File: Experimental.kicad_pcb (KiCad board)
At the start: 4 copper layers, 50.5 x 71 mm, 64 parts, among them J1 3v3 Terminal, J2 Screw_Terminal, J3 Screw_Terminal_4x, J4 Screw_Terminal_4x, J5 -/+ LIPO PIN, J6 Screw_Terminal, J7 20279-001E-03, J8 GND Terminal, Q1 AO3400A, Q2_32mW1 AO3400A, Q4 AO3400A, U6 NEO-6M-GPS

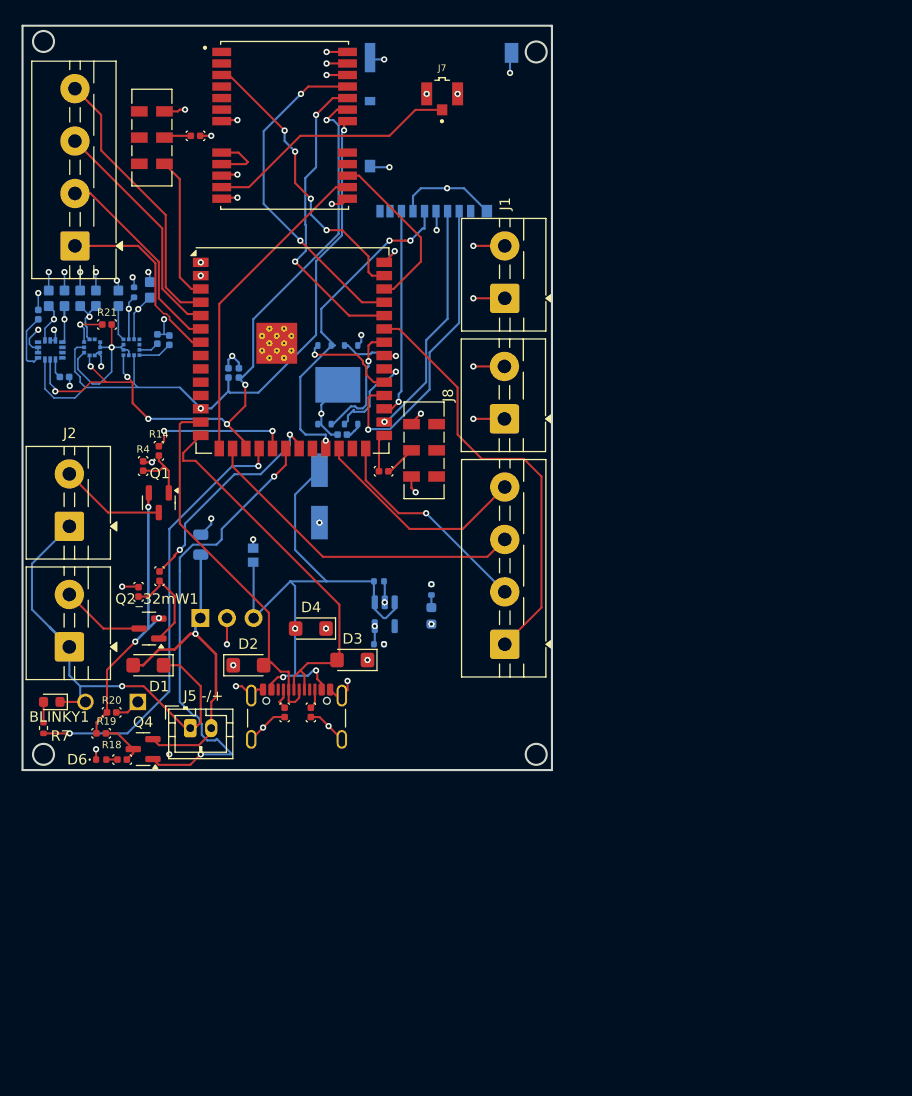
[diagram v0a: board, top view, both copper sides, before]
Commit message: Version 4.0
Schematic Cleanup and PCB Layout/Impletementation
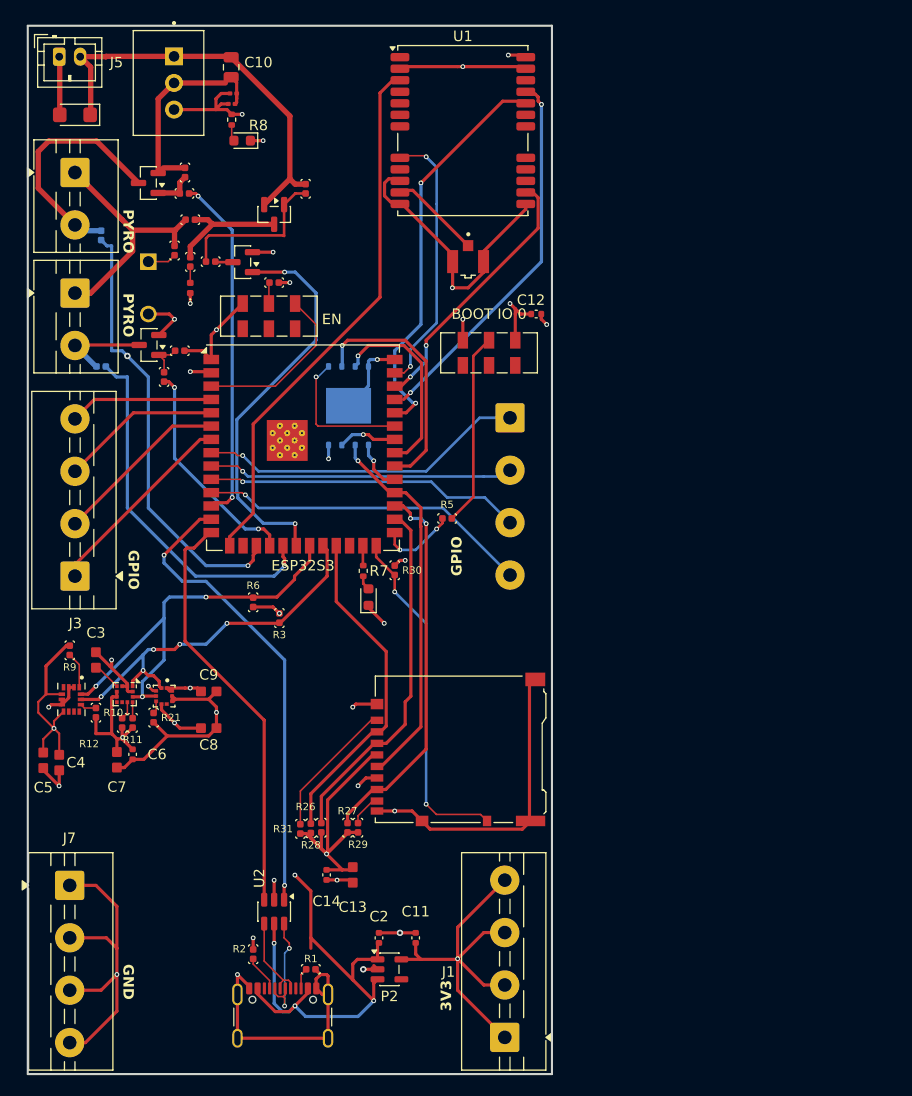
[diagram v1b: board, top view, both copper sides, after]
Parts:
- removed 5v1: LP5907MFX-3.3, Package_TO_SOT_SMD:SOT-23-5
- removed BLINKY1: GREEN LED, LED_SMD:LED_0603_1608Metric
- removed D3: SMF6V0A, Diode_SMD:D_SMF
- removed D4: SMF6V5A, Diode_SMD:D_SMF
- removed D6: RED LED, LED_SMD:LED_0402_1005Metric
- removed J4: Screw_Terminal_4x, TerminalBlock:TerminalBlock_MaiXu_MX126-5.0-04P_1x04_P5.00mm
- removed J5 -/+: LIPO PIN, Connector_JST:JST_PH_B2B-PH-K_1x02_P2.00mm_Vertical
- removed J6: Screw_Terminal, TerminalBlock:TerminalBlock_MaiXu_MX126-5.0-02P_1x02_P5.00mm
- removed J8: GND Terminal, TerminalBlock:TerminalBlock_MaiXu_MX126-5.0-02P_1x02_P5.00mm
- removed OnLight1: RED_LED, LED_SMD:LED_0603_1608Metric
- removed Q2_32mW1: AO3400A, Package_TO_SOT_SMD:SOT-23
- removed R13: 10k, Resistor:R0402
- removed U6: NEO-6M-GPS, footprints:XCVR_NEO-6M-GPS
- added C12: 100nf, Capacitor_SMD:C_0402_1005Metric, F.Cu at (149.0, 77.5)
- added C12_47uF1: 06034W476MAT2A, Capacitor_SMD:C_0201_0603Metric, F.Cu at (120.1, 56.5)
- added C12_47uF2: 06034W476MAT2A, Capacitor_SMD:C_0201_0603Metric, F.Cu at (120.0, 57.5)
- added GREEN_LED1: NCD0603G1, LED_SMD:LED_0603_1608Metric, F.Cu at (133.0, 104.5)
- added J10: Screw_Terminal, TerminalBlock:TerminalBlock_MaiXu_MX126-5.0-02P_1x02_P5.00mm, F.Cu at (105.0, 64.0)
- added J5: LIPO PIN, Connector_JST:JST_PH_B2B-PH-K_1x02_P2.00mm_Vertical, F.Cu at (103.5, 53.0)
- added J7CHECK1: 20279-001E-03, footprints:IPEX_20279-001E-03, F.Cu at (142.5, 72.5)
- added J9: MX128-5.0-04P-GN01-Cu-Y-A, TerminalBlock:TerminalBlock_MaiXu_MX126-5.0-04P_1x04_P5.00mm, B.Cu at (146.5, 87.4)
- added NCD0603R1: RED_LED, LED_SMD:LED_0603_1608Metric, F.Cu at (121.0, 61.0)
- added P2: LP5907MFX-3.3, Package_TO_SOT_SMD:SOT-23-5, F.Cu at (135.0, 140.0)
- added Q2: AO3400A, Package_TO_SOT_SMD:SOT-23, F.Cu at (112.1, 80.5)
- added Q3: AO3400A, Package_TO_SOT_SMD:SOT-23, F.Cu at (121.0, 72.5)
- added R22: 147, Resistor:R0402, F.Cu at (114.5, 71.4)
- added R23: 1 ohm, 20W, Resistor:R0402, F.Cu at (116.0, 68.5)
- added R24: 10k, Resistor:R0402, F.Cu at (127.0, 65.6)
- added R25: 2200, Resistor:R0402, F.Cu at (117.9, 72.5)
- added R26: 10k, Resistor:R0402, F.Cu at (128.5, 126.5)
- added R27: 10k, Resistor:R0402, F.Cu at (131.0, 126.5)
- added R28: 10k, Resistor:R0402, F.Cu at (127.5, 126.6)
- added R29: 10k, Resistor:R0402, F.Cu at (132.0, 126.5)
- added R30: 10k, Resistor:R0402, F.Cu at (135.5, 101.9)
- added R31: 10k, Resistor:R0402, F.Cu at (126.5, 126.6)
- added U1: NEO-M8N, RF_GPS:ublox_NEO, F.Cu at (142.0, 60.0)
- added U2: USBLC6-2SC6, Package_TO_SOT_SMD:SOT-23-6, F.Cu at (124.0, 134.5)
- Barometer1, C10, C2, C3, C4, C5, C6, C7, C8, C9, PS1, R10, R11, R12, R3, R6, R8, R9, SDCard1: moved to F.Cu
- C1: value 1uf -> 6800 UF; footprint Capacitor_SMD:C_0402_1005Metric -> Capacitor:CAPPRD500W85D1250H3700
- C11: value 47uF 3.037mOhm -> 1uf; footprint Capacitor:EEEHP1H4R7P -> Capacitor_SMD:C_0402_1005Metric; moved to F.Cu
- C13: value 06034W476MAT2A -> 100nF; footprint Capacitor:CAPC1608X100N -> Capacitor:CAPC1608X90N; moved to F.Cu
- C14: value 6800 UF -> 10uF; footprint Capacitor:CAPPRD500W85D1250H3700 -> Capacitor_SMD:C_0402_1005Metric; moved to F.Cu
- D2: value SMF6V0A -> RED LED; footprint Diode_SMD:D_SMF -> LED_SMD:LED_0402_1005Metric
- ESP32S3: value ESP32-S3-WROOM-1U -> ESP32-S3-WROOM-1U-N4
- IMU6axis1: value LSM6DSOX -> LSM6DSOXTR; moved to F.Cu
- J1: value 3v3 Terminal -> MX128-5.0-04P-GN01-Cu-Y-A; footprint TerminalBlock:TerminalBlock_MaiXu_MX126-5.0-02P_1x02_P5.00mm -> TerminalBlock:TerminalBlock_MaiXu_MX126-5.0-04P_1x04_P5.00mm
- J3: value Screw_Terminal_4x -> MX128-5.0-04P-GN01-Cu-Y-A
- J7: value 20279-001E-03 -> MX128-5.0-04P-GN01-Cu-Y-A; footprint footprints:IPEX_20279-001E-03 -> TerminalBlock:TerminalBlock_MaiXu_MX126-5.0-04P_1x04_P5.00mm
- Magnometer1: value LIS3MDL -> LIS3MDLTR; moved to F.Cu
- Q4: value AO3400A -> FDN340P
- R14: value 330 -> 10k; moved to B.Cu
- R16: value 330 -> 10k
- R18: value 10k -> 330
- R19: value 1 ohm, 20W -> 330
- R20: value 147 -> 10k
- R4: moved to B.Cu
- moved J7 83.4 mm to (104.5, 132.0), turned to -90 degrees
- moved J1 70.5 mm to (146.0, 146.5)
- moved SDCard1 59.1 mm to (141.5, 119.0), turned to 90 degrees
- moved R18 54.3 mm to (115.4, 66.0), turned to -90 degrees
- moved D1 53.0 mm to (105.0, 58.5)
- moved Q4 52.5 mm to (124.0, 68.0), turned to -90 degrees
- moved PS1 51.3 mm to (114.5, 55.5), turned to -90 degrees
- moved R8 48.7 mm to (120.0, 59.0)
- moved C10 45.6 mm to (119.9, 54.0), turned to 90 degrees
- moved C7 44.9 mm to (109.0, 120.0), turned to -90 degrees
- moved C4 44.3 mm to (103.5, 120.3), turned to 90 degrees
- moved C5 44.1 mm to (102.0, 120.1), turned to 90 degrees
- moved C6 44.1 mm to (110.5, 119.5), turned to -90 degrees
- moved R20 43.6 mm to (116.0, 72.5), turned to 180 degrees
- moved C11 43.1 mm to (137.5, 137.0), turned to -90 degrees
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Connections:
- net /Storage/CMD renamed Net-(ESP32S3-IO35)
- net /Storage/DAT0 renamed Net-(ESP32S3-IO36)
- net /Storage/Digital_IN renamed Net-(ESP32S3-IO38)
- net /Storage/Digital_OUT renamed Net-(ESP32S3-IO39)
- Barometer1 pad 2: /NEO-6M-GPS/SCL -> Net-(Barometer1-SCK)
- Barometer1 pad 4: /NEO-6M-GPS/SDA -> Net-(Barometer1-SDI)
- C1 pad 1: GND -> Net-(C1-+)
- C1 pad 2: +5V -> GND
- C11 pad 2: +5V -> +3V3
- C13 pad 2: +5V -> +3V3
- C14 pad 1: Net-(C14-+) -> GND
- C14 pad 2: GND -> +3V3
- C2 pad 2: +3V3 -> +5V
- D1 pad 1: GND -> +7.4V
- D1 pad 2: +7.4V -> GND
- D2 pad 2: /USB_C_PORT/USB_D- -> Net-(D2-A)
- ESP32S3 pad 10: unconnected-(ESP32S3-IO17-Pad10) -> Net-(ESP32S3-IO17)
- ESP32S3 pad 11: unconnected-(ESP32S3-IO18-Pad11) -> Net-(ESP32S3-IO18)
- ESP32S3 pad 12: /NEO-6M-GPS/SDA -> /PYRO2_FIRE
- ESP32S3 pad 13: /USB_C_PORT/USB_D- -> Net-(ESP32S3-IO19)
- ESP32S3 pad 14: /USB_C_PORT/USB_D+ -> Net-(ESP32S3-IO20)
- ESP32S3 pad 15: /NEO-6M-GPS/GPS_MOSI -> Net-(ESP32S3-IO3)
- ESP32S3 pad 16: Net-(ESP32S3-IO46) -> unconnected-(ESP32S3-IO46-Pad16)
- ESP32S3 pad 17: /NEO-6M-GPS/SCL -> GND
- ESP32S3 pad 18: /POWER_MANAGEMENT/LED -> /PYRO_FIRE
- ESP32S3 pad 19: /PYRO_N_MOSFET_A1/Pyro2 -> GND
- ESP32S3 pad 20: /PYRO_N_MOSFET_A1/Charge_Pyro -> /CHARGE_PYRO
- ESP32S3 pad 21: /PYRO_N_MOSFET_A1/Pyro -> Net-(Barometer1-SDI)
- ESP32S3 pad 22: unconnected-(ESP32S3-IO14-Pad22) -> Net-(Barometer1-SCK)
- ESP32S3 pad 23: /Storage/CLK -> Net-(ESP32S3-IO21)
- ESP32S3 pad 24: Net-(ESP32S3-IO47) -> unconnected-(ESP32S3-IO47-Pad24)
- ESP32S3 pad 25: unconnected-(ESP32S3-IO48-Pad25) -> Net-(ESP32S3-IO48)
- ESP32S3 pad 26: Net-(ESP32S3-IO45) -> /DET_A
- ESP32S3 pad 30: /Storage/DAT3/CD -> Net-(ESP32S3-IO37)
- ESP32S3 pad 33: /Storage/HOLD/RESET -> Net-(ESP32S3-IO40)
- ESP32S3 pad 34: /Storage/WP -> Net-(ESP32S3-IO41)
- ESP32S3 pad 35: Net-(ESP32S3-IO42) -> /CS_FLASH
- ESP32S3 pad 36: /NEO-6M-GPS/GPS_TXD1 -> Net-(ESP32S3-RXD0)
- ESP32S3 pad 37: /NEO-6M-GPS/GPS_RXD1 -> Net-(ESP32S3-TXD0)
- ESP32S3 pad 38: /NEO-6M-GPS/GPS_MISO -> Net-(ESP32S3-IO2)
- ESP32S3 pad 39: /NEO-6M-GPS/TIMEPULSE -> /~{RESET}
- ESP32S3 pad 8: unconnected-(ESP32S3-IO15-Pad8) -> Net-(ESP32S3-IO15)
- ESP32S3 pad 9: unconnected-(ESP32S3-IO16-Pad9) -> Net-(ESP32S3-IO16)
- IMU6axis1 pad 13: /NEO-6M-GPS/SCL -> Net-(Barometer1-SCK)
- IMU6axis1 pad 14: /NEO-6M-GPS/SDA -> Net-(Barometer1-SDI)
- J2 pad 1: GND -> Net-(J10-Pin_1)
- J7 pad 1: Net-(U6-RF_IN) -> GND
- Magnometer1 pad 1: /NEO-6M-GPS/SCL -> Net-(Barometer1-SCK)
- Magnometer1 pad 11: /NEO-6M-GPS/SDA -> Net-(Barometer1-SDI)
- PowerUpload1 pad A6: /USB_C_PORT/USB_D+ -> Net-(PowerUpload1-D+-PadA6)
- PowerUpload1 pad A7: /USB_C_PORT/USB_D- -> Net-(PowerUpload1-D--PadA7)
- PowerUpload1 pad B6: /USB_C_PORT/USB_D+ -> Net-(PowerUpload1-D+-PadA6)
- PowerUpload1 pad B7: /USB_C_PORT/USB_D- -> Net-(PowerUpload1-D--PadA7)
- Q1 pad 2: Net-(Q1-S) -> GND
- Q1 pad 3: Net-(J2-Pin_2) -> Net-(J10-Pin_2)
- Q4 pad 1: /PYRO_N_MOSFET_A1/Charge_Pyro -> Net-(Q4-G)
- R14 pad 1: /PYRO_N_MOSFET_A1/Pyro2 -> GND
- R14 pad 2: Net-(Q1-G) -> Net-(J2-Pin_2)
- R15 pad 2: Net-(Q2_32mW1-G) -> Net-(Q1-G)
- R16 pad 1: /PYRO_N_MOSFET_A1/Pyro -> GND
- R16 pad 2: Net-(Q2_32mW1-G) -> Net-(Q2-G)
- R18 pad 1: Net-(D6-A) -> /PYRO2_FIRE
- R18 pad 2: Net-(Q4-D) -> Net-(Q1-G)
- R19 pad 1: Net-(Q1-S) -> /PYRO_FIRE
- R19 pad 2: Net-(Q4-D) -> Net-(Q2-G)
- R20 pad 1: Net-(C14-+) -> Net-(D2-A)
- R20 pad 2: Net-(Q1-S) -> Net-(Q4-D)
- R3 pad 1: /NEO-6M-GPS/SCL -> Net-(Barometer1-SCK)
- R4 pad 2: Net-(Q1-G) -> Net-(J10-Pin_2)
- R6 pad 1: /NEO-6M-GPS/SDA -> Net-(Barometer1-SDI)
- R7 pad 1: /POWER_MANAGEMENT/LED -> Net-(ESP32S3-IO48)
- R8 pad 1: +3V3 -> +5V
- SDCard1 pad 1: unconnected-(SDCard1-DAT2-Pad1) -> Net-(SDCard1-DAT2)
- SDCard1 pad 10: unconnected-(SDCard1-DET_A-Pad10) -> /DET_A
- SDCard1 pad 2: /Storage/DAT3/CD -> Net-(ESP32S3-IO21)
- SDCard1 pad 5: /Storage/CLK -> Net-(ESP32S3-IO37)
- SDCard1 pad 8: unconnected-(SDCard1-DAT1-Pad8) -> Net-(SDCard1-DAT1)
- SDCard1 pad 9: unconnected-(SDCard1-DET_B-Pad9) -> GND
- WSON-8-Flash1 pad 1: Net-(WSON-8-Flash1-~{CS}) -> /CS_FLASH
- WSON-8-Flash1 pad 3: /Storage/WP -> Net-(ESP32S3-IO40)
- WSON-8-Flash1 pad 6: /Storage/CLK -> Net-(ESP32S3-IO37)
- WSON-8-Flash1 pad 7: /Storage/HOLD/RESET -> Net-(ESP32S3-IO41)
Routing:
- net GND: track 143.6 -> 305.2 mm, vias 46 -> 27
- net +3V3: track 50.3 -> 135.1 mm, vias 21 -> 13
- net +5V: track 53.6 -> 135.5 mm, vias 3 -> 5
- net /NEO-6M-GPS/SCL: track 69.4 -> 0.00 mm, vias 7 -> 0
- net /NEO-6M-GPS/SDA: track 64.4 -> 0.00 mm, vias 2 -> 0
- net Net-(ESP32S3-IO3): track 0.00 -> 51.6 mm
- net /PYRO_N_MOSFET_A1/Charge_Pyro: track 45.8 -> 0.00 mm, vias 2 -> 0
- net Net-(ESP32S3-IO19): track 0.00 -> 44.9 mm, vias 0 -> 2
- net /POWER_MANAGEMENT/LED: track 41.8 -> 0.00 mm, vias 2 -> 0
- net Net-(ESP32S3-IO42): track 40.9 -> 0.00 mm
- net Net-(Barometer1-SDI): track 0.00 -> 40.2 mm, vias 0 -> 3
- net Net-(ESP32S3-IO20): track 0.00 -> 39.7 mm
- net Net-(ESP32S3-RXD0): track 0.00 -> 38.6 mm, vias 0 -> 2
- net /CHARGE_PYRO: track 0.00 -> 38.2 mm, vias 0 -> 2
- net Net-(Barometer1-SCK): track 0.00 -> 37.6 mm, vias 0 -> 5
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- added copper zone on In2.Cu, net +3V3
- added copper zone on In1.Cu, net GND
- removed copper zone on In1.Cu, net +3V3
- removed copper zone on In2.Cu, net GND
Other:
- board size 50.5 x 71 mm -> 50 x 100 mm
- board text added: "3V3"
- board text added: "BOOT IO 0"
- board text added: "EN"
- board text added: "GND"
- board text added: "GPIO"
- board text added: "PYRO"

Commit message: Version 5.0!
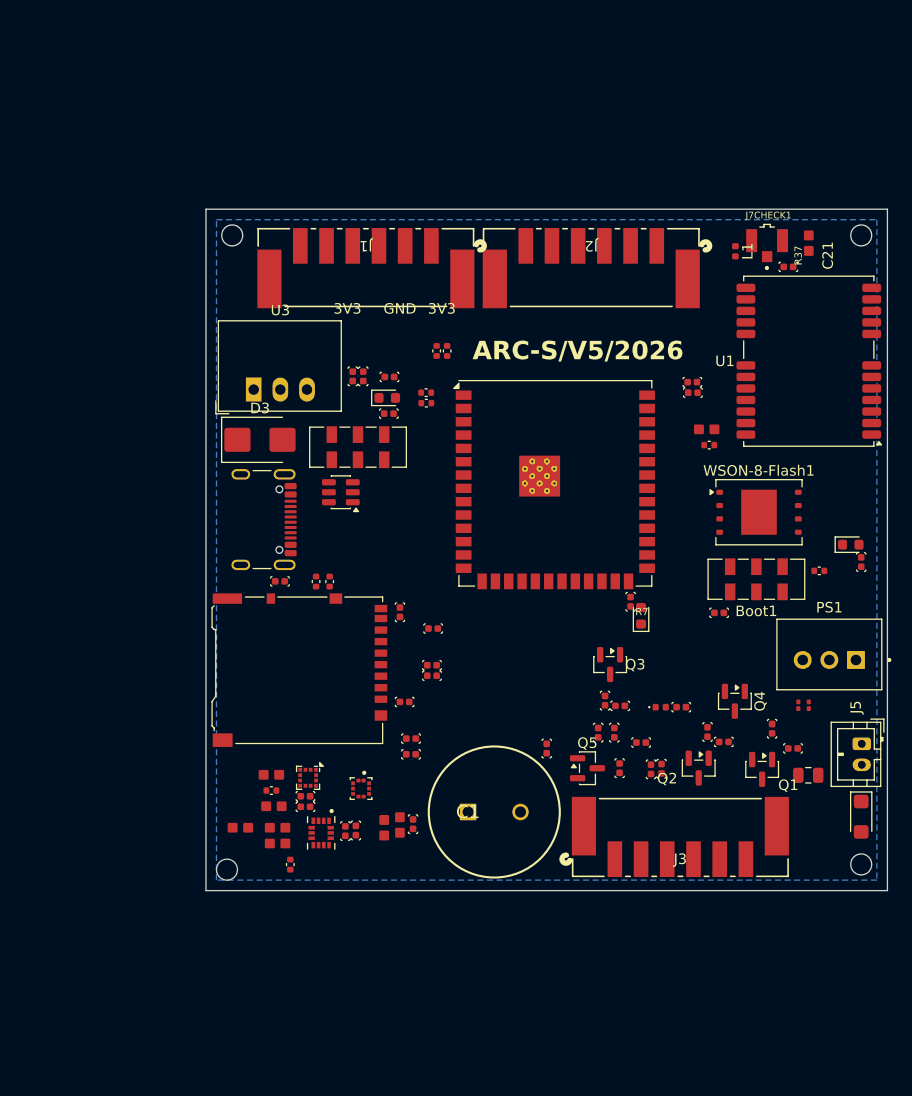
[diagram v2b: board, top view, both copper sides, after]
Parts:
- removed GREEN_LED1: NCD0603G1, LED_SMD:LED_0603_1608Metric
- removed J10: Screw_Terminal, TerminalBlock:TerminalBlock_MaiXu_MX126-5.0-02P_1x02_P5.00mm
- removed J7, J9: MX128-5.0-04P-GN01-Cu-Y-A, TerminalBlock:TerminalBlock_MaiXu_MX126-5.0-04P_1x04_P5.00mm
- removed P2: LP5907MFX-3.3, Package_TO_SOT_SMD:SOT-23-5
- added BLUE_LED1: NCD0603G1, LED_SMD:LED_0603_1608Metric, F.Cu at (159.0, 106.3)
- added C15: 100nF, Capacitor:CAPC1608X90N, F.Cu at (165.3, 88.5)
- added C16: 10uF, Capacitor_SMD:C_0402_1005Metric, F.Cu at (165.5, 90.0)
- added C17: 10uF, Capacitor_SMD:C_0402_1005Metric, F.Cu at (138.5, 85.0)
- added C18: 10uF, Capacitor_SMD:C_0402_1005Metric, F.Cu at (140.5, 81.0)
- added C19: 1uf, Capacitor_SMD:C_0402_1005Metric, F.Cu at (138.5, 86.0)
- added C20: 1uf, Capacitor_SMD:C_0402_1005Metric, F.Cu at (139.5, 81.0)
- added C21: 10nF, Capacitor:CAPC1608X90N, F.Cu at (175.0, 70.7)
- added D3: B220, Diode_SMD:D_SMB, F.Cu at (122.7, 89.5)
- added L1: 27 nH, Inductor_SMD:L_0402_1005Metric, F.Cu at (168.0, 71.5)
- added NCD0603R2: RED_LED, LED_SMD:LED_0603_1608Metric, F.Cu at (134.8, 85.5)
- added Q5: AO3400A, Package_TO_SOT_SMD:SOT-23, F.Cu at (153.9, 120.8)
- added R13: 30, Resistor:R0402, F.Cu at (163.9, 84.0)
- added R32: 30, Resistor:R0402, F.Cu at (163.9, 85.0)
- added R33: 1k, Resistor:R0402, F.Cu at (134.9, 87.0)
- added R34: 330, Resistor:R0402, F.Cu at (154.9, 117.4)
- added R35: 10k, Resistor:R0402, F.Cu at (156.4, 117.4)
- added R36: 10k, Resistor:R0402, F.Cu at (150.0, 118.9)
- added R37: 10, Resistor:R0402, F.Cu at (173.1, 73.0)
- added U3: R-783.3-1.0, Converter_DCDC:Converter_DCDC_RECOM_R-78E-0.5_THT, F.Cu at (122.1, 84.7)
- C1, R14, R4, WSON-8-Flash1: moved to F.Cu
- J1, J3: value MX128-5.0-04P-GN01-Cu-Y-A -> SPRING_CONN; footprint TerminalBlock:TerminalBlock_MaiXu_MX126-5.0-04P_1x04_P5.00mm -> footprints:6P_SMD_SPRING_CONN
- J2: value Screw_Terminal -> SPRING_CONN; footprint TerminalBlock:TerminalBlock_MaiXu_MX126-5.0-02P_1x02_P5.00mm -> footprints:6P_SMD_SPRING_CONN
- NCD0603R1: value RED_LED -> GREEN_LED
- R7: value 5.4k -> 1k; footprint Resistor_SMD:R_0402_1005Metric -> Resistor:R0402
- R8: value 5.4k -> 330; footprint Resistor_SMD:R_0402_1005Metric -> Resistor:R0402
- moved J5 100.8 mm to (180.1, 118.5), turned to -90 degrees
- moved D1 100.5 mm to (180.0, 125.5), turned to -90 degrees
- moved C10 87.1 mm to (174.9, 121.5), turned to 0 degrees
- moved PS1 83.3 mm to (177.0, 110.5), turned to 180 degrees
- moved Q1 81.0 mm to (170.6, 120.9), turned to -90 degrees
- moved R15 79.9 mm to (173.5, 118.9), turned to -90 degrees
- moved C12_47uF2 79.5 mm to (175.0, 114.8), turned to 90 degrees
- moved C12_47uF1 79.4 mm to (174.0, 114.8), turned to 90 degrees
- moved R18 75.8 mm to (171.5, 117.1), turned to 0 degrees
- moved J1 74.6 mm to (132.8, 73.1), turned to 180 degrees
- moved R8 73.4 mm to (180.0, 101.2), turned to 180 degrees
- moved R4 73.1 mm to (159.9, 120.9)
- moved NCD0603R1 69.7 mm to (179.0, 99.5), turned to 0 degrees
- moved Q2 66.2 mm to (164.5, 120.8), turned to -90 degrees
- moved R23 65.9 mm to (159.0, 118.4)
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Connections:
- Barometer1 pad 2: Net-(Barometer1-SCK) -> /SCL
- Barometer1 pad 4: Net-(Barometer1-SDI) -> /SDA
- Boot2 pad 1: GND -> Net-(Boot2A-A)
- Boot2 pad 2: Net-(Boot2A-B) -> +5V
- C2 pad 2: +5V -> Net-(Boot2A-A)
- C3 pad 1: Net-(Magnometer1-C1) -> GND
- C3 pad 2: GND -> Net-(Magnometer1-C1)
- C8 pad 1: +3V3 -> GND
- C8 pad 2: GND -> +3V3
- C9 pad 1: +3V3 -> GND
- C9 pad 2: GND -> +3V3
- ESP32S3 pad 10: Net-(ESP32S3-IO17) -> /D-
- ESP32S3 pad 12: /PYRO2_FIRE -> /Pad12_CMD
- ESP32S3 pad 14: Net-(ESP32S3-IO20) -> /DET_A
- ESP32S3 pad 16: unconnected-(ESP32S3-IO46-Pad16) -> /SCL
- ESP32S3 pad 17: GND -> /SDA
- ESP32S3 pad 18: /PYRO_FIRE -> /PYRO1_CONTINUITY
- ESP32S3 pad 19: GND -> /PYRO1_FIRE
- ESP32S3 pad 20: /CHARGE_PYRO -> /PYRO2_CONTINUITY
- ESP32S3 pad 21: Net-(Barometer1-SDI) -> /PYRO2_FIRE
- ESP32S3 pad 22: Net-(Barometer1-SCK) -> /PYRO3_CONTINUITY
- ESP32S3 pad 23: Net-(ESP32S3-IO21) -> /PYRO3_FIRE
- ESP32S3 pad 24: unconnected-(ESP32S3-IO47-Pad24) -> /CHARGE_PYRO
- ESP32S3 pad 25: Net-(ESP32S3-IO48) -> unconnected-(ESP32S3-IO48-Pad25)
- ESP32S3 pad 26: /DET_A -> Net-(ESP32S3-IO45)
- ESP32S3 pad 28: Net-(ESP32S3-IO35) -> /CLK
- ESP32S3 pad 3: Net-(Boot2A-C) -> Net-(ESP32S3-EN)
- ESP32S3 pad 34: Net-(ESP32S3-IO41) -> unconnected-(ESP32S3-IO41-Pad34)
- ESP32S3 pad 35: /CS_FLASH -> /~{RESET}
- ESP32S3 pad 39: /~{RESET} -> Net-(ESP32S3-IO1)
- ESP32S3 pad 8: Net-(ESP32S3-IO15) -> /Pad_8
- ESP32S3 pad 9: Net-(ESP32S3-IO16) -> /D+
- IMU6axis1 pad 13: Net-(Barometer1-SCK) -> /SCL
- IMU6axis1 pad 14: Net-(Barometer1-SDI) -> /SDA
- J1 pad 1: +3V3 -> Net-(ESP32S3-IO3)
- J1 pad 2: +3V3 -> Net-(ESP32S3-IO4)
- J1 pad 3: +3V3 -> Net-(ESP32S3-IO5)
- J1 pad 4: +3V3 -> Net-(ESP32S3-IO6)
- J2 pad 1: Net-(J10-Pin_1) -> +3V3
- J2 pad 2: Net-(J2-Pin_2) -> GND
- J3 pad 1: Net-(ESP32S3-IO7) -> Net-(Q5-D)
- J3 pad 2: Net-(ESP32S3-IO6) -> Net-(J3-Pad2)
- J3 pad 3: Net-(ESP32S3-IO5) -> Net-(Q2-D)
- J3 pad 4: Net-(ESP32S3-IO4) -> Net-(J3-Pad2)
- Magnometer1 pad 1: Net-(Barometer1-SCK) -> /SCL
- Magnometer1 pad 11: Net-(Barometer1-SDI) -> /SDA
- PowerUpload1 pad A4: +5V -> Net-(D3-A)
- PowerUpload1 pad A9: +5V -> Net-(D3-A)
- PowerUpload1 pad B4: +5V -> Net-(D3-A)
- PowerUpload1 pad B9: +5V -> Net-(D3-A)
- Q1 pad 3: Net-(J10-Pin_2) -> Net-(Q1-D)
- Q2 pad 3: Net-(J2-Pin_2) -> Net-(Q2-D)
- R14 pad 1: GND -> /PYRO2_CONTINUITY
- R14 pad 2: Net-(J2-Pin_2) -> Net-(Q2-D)
- R17 pad 1: Net-(Boot2A-B) -> Net-(ESP32S3-EN)
- R18 pad 1: /PYRO2_FIRE -> /PYRO3_FIRE
- R19 pad 1: /PYRO_FIRE -> /PYRO2_FIRE
- R22 pad 2: Net-(J10-Pin_1) -> Net-(J3-Pad2)
- R23 pad 1: Net-(J10-Pin_1) -> Net-(J3-Pad2)
- R26 pad 2: Net-(ESP32S3-IO35) -> /Pad12_CMD
- R27 pad 1: Net-(ESP32S3-IO36) -> Net-(ESP32S3-IO19)
- R28 pad 1: Net-(ESP32S3-IO21) -> Net-(ESP32S3-IO18)
- R3 pad 1: Net-(Barometer1-SCK) -> /SCL
- R4 pad 1: GND -> /PYRO3_CONTINUITY
- R4 pad 2: Net-(J10-Pin_2) -> Net-(Q1-D)
- R6 pad 1: Net-(Barometer1-SDI) -> /SDA
- R7 pad 1: Net-(ESP32S3-IO48) -> Net-(ESP32S3-IO45)
- SDCard1 pad 2: Net-(ESP32S3-IO21) -> Net-(ESP32S3-IO18)
- SDCard1 pad 3: Net-(ESP32S3-IO35) -> /Pad12_CMD
- SDCard1 pad 5: Net-(ESP32S3-IO37) -> /CLK
- SDCard1 pad 7: Net-(ESP32S3-IO36) -> Net-(ESP32S3-IO19)
- U1 pad 14: Net-(ESP32S3-IO2) -> Net-(ESP32S3-IO1)
- U1 pad 20: Net-(ESP32S3-RXD0) -> Net-(U1-TXD/SPI_MISO)
- U1 pad 21: Net-(ESP32S3-TXD0) -> Net-(U1-RXD/SPI_MOSI)
- U1 pad 3: Net-(ESP32S3-IO3) -> Net-(ESP32S3-IO2)
- U1 pad 9: unconnected-(U1-VCC_RF-Pad9) -> Net-(U1-VCC_RF)
- U2 pad 1: Net-(ESP32S3-IO19) -> /D-
- U2 pad 3: Net-(ESP32S3-IO20) -> /D+
- U2 pad 5: +5V -> Net-(Boot2A-A)
- WSON-8-Flash1 pad 1: /CS_FLASH -> Net-(ESP32S3-IO36)
- WSON-8-Flash1 pad 2: Net-(ESP32S3-IO39) -> Net-(ESP32S3-IO37)
- WSON-8-Flash1 pad 3: Net-(ESP32S3-IO40) -> Net-(ESP32S3-IO38)
- WSON-8-Flash1 pad 5: Net-(ESP32S3-IO38) -> Net-(ESP32S3-IO39)
- WSON-8-Flash1 pad 6: Net-(ESP32S3-IO37) -> /CLK
- WSON-8-Flash1 pad 7: Net-(ESP32S3-IO41) -> Net-(ESP32S3-IO40)
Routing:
- net GND: track 305.2 -> 0.00 mm, vias 27 -> 0
- net +5V: track 135.5 -> 0.00 mm, vias 5 -> 0
- net +3V3: track 135.1 -> 0.00 mm, vias 13 -> 0
- net Net-(ESP32S3-IO3): track 51.6 -> 0.00 mm
- net Net-(ESP32S3-IO19): track 44.9 -> 0.00 mm, vias 2 -> 0
- net Net-(Barometer1-SDI): track 40.2 -> 0.00 mm, vias 3 -> 0
- net Net-(ESP32S3-IO20): track 39.7 -> 0.00 mm
- net +7.4V: track 39.6 -> 0.00 mm
- net Net-(ESP32S3-RXD0): track 38.6 -> 0.00 mm, vias 2 -> 0
- net /CHARGE_PYRO: track 38.2 -> 0.00 mm, vias 2 -> 0
- net Net-(Barometer1-SCK): track 37.6 -> 0.00 mm, vias 5 -> 0
- net Net-(ESP32S3-IO36): track 36.4 -> 0.00 mm, vias 2 -> 0
- net Net-(ESP32S3-IO37): track 36.1 -> 0.00 mm, vias 1 -> 0
- net Net-(ESP32S3-TXD0): track 35.9 -> 0.00 mm, vias 2 -> 0
- net Net-(ESP32S3-IO35): track 34.1 -> 0.00 mm
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- added copper zone on B.Cu, net GND
- removed copper zone on In2.Cu, net +3V3
- removed copper zone on In1.Cu, net GND
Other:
- board size 50 x 100 mm -> 65 x 65 mm
- copper layers 4 -> 2
- board text added: "ARC-S/V5/2026"
- board text removed: "BOOT IO 0"
- board text removed: "EN"
- board text removed: "GPIO"
- board text removed: "PYRO"
